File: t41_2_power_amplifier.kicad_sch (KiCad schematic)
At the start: 45 parts, among them J1 5-1814832-1, J2 5-1814832-1, J3 B2B-XH-A_LF__SN_, J5 Screw_Terminal_01x02, Q1 Q_NMOS_GSD, Q3 Q_NMOS_GSD, T1 Transformer_1P_SS, T2 Transformer_1P_1S, U1 MCP1802x-xx02xOT

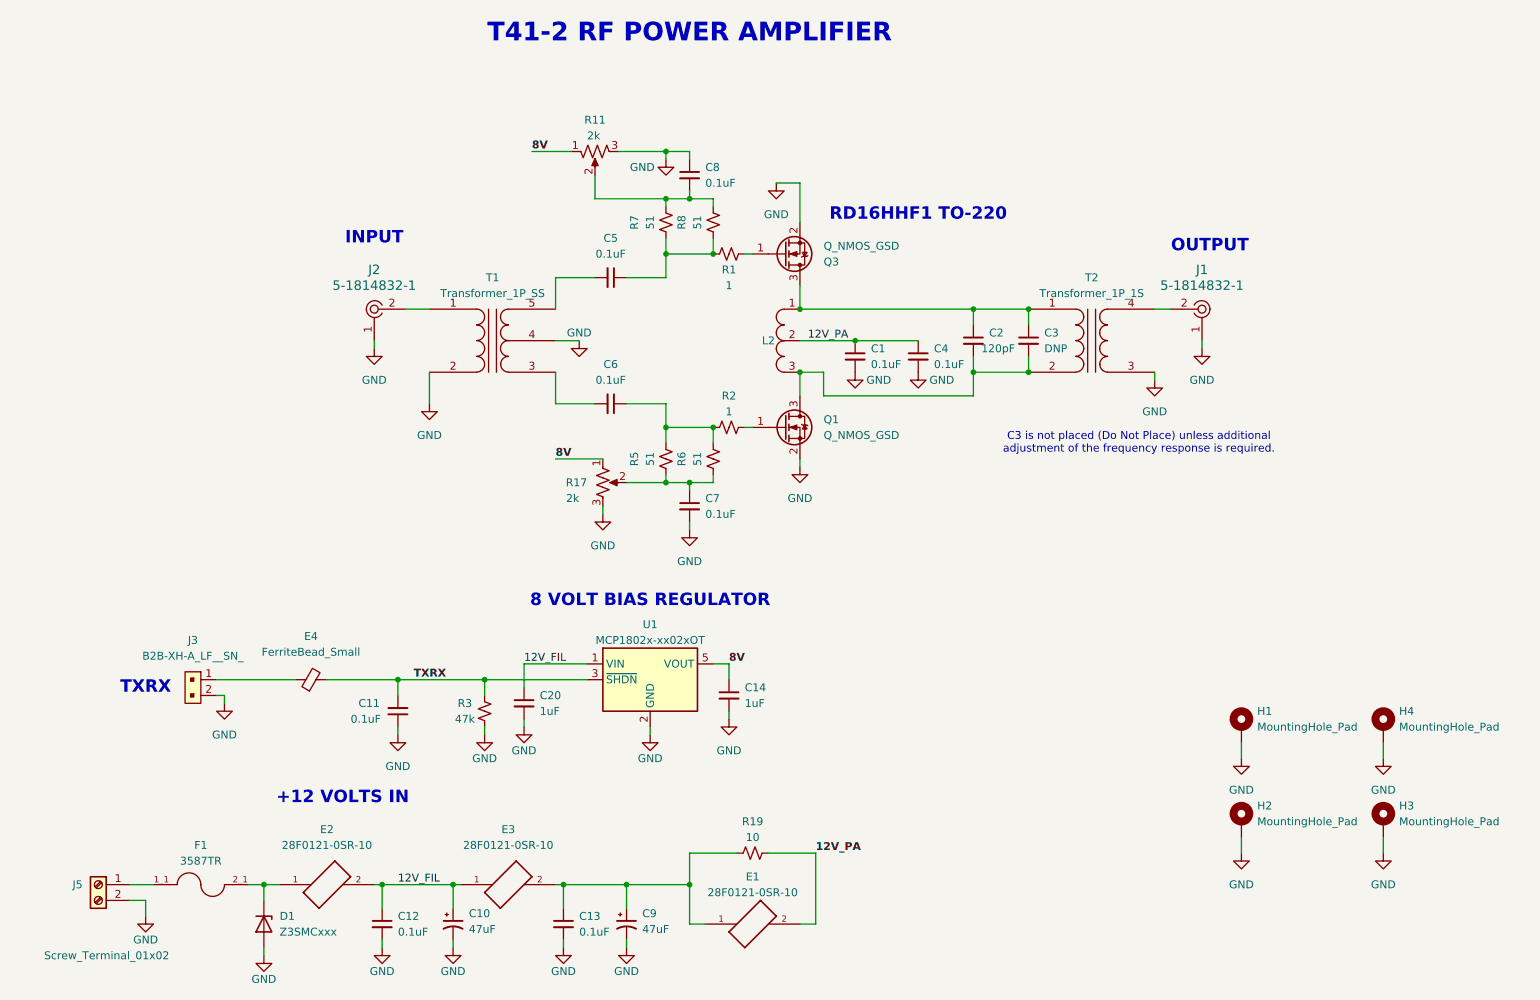
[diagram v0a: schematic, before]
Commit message: Added zip files.
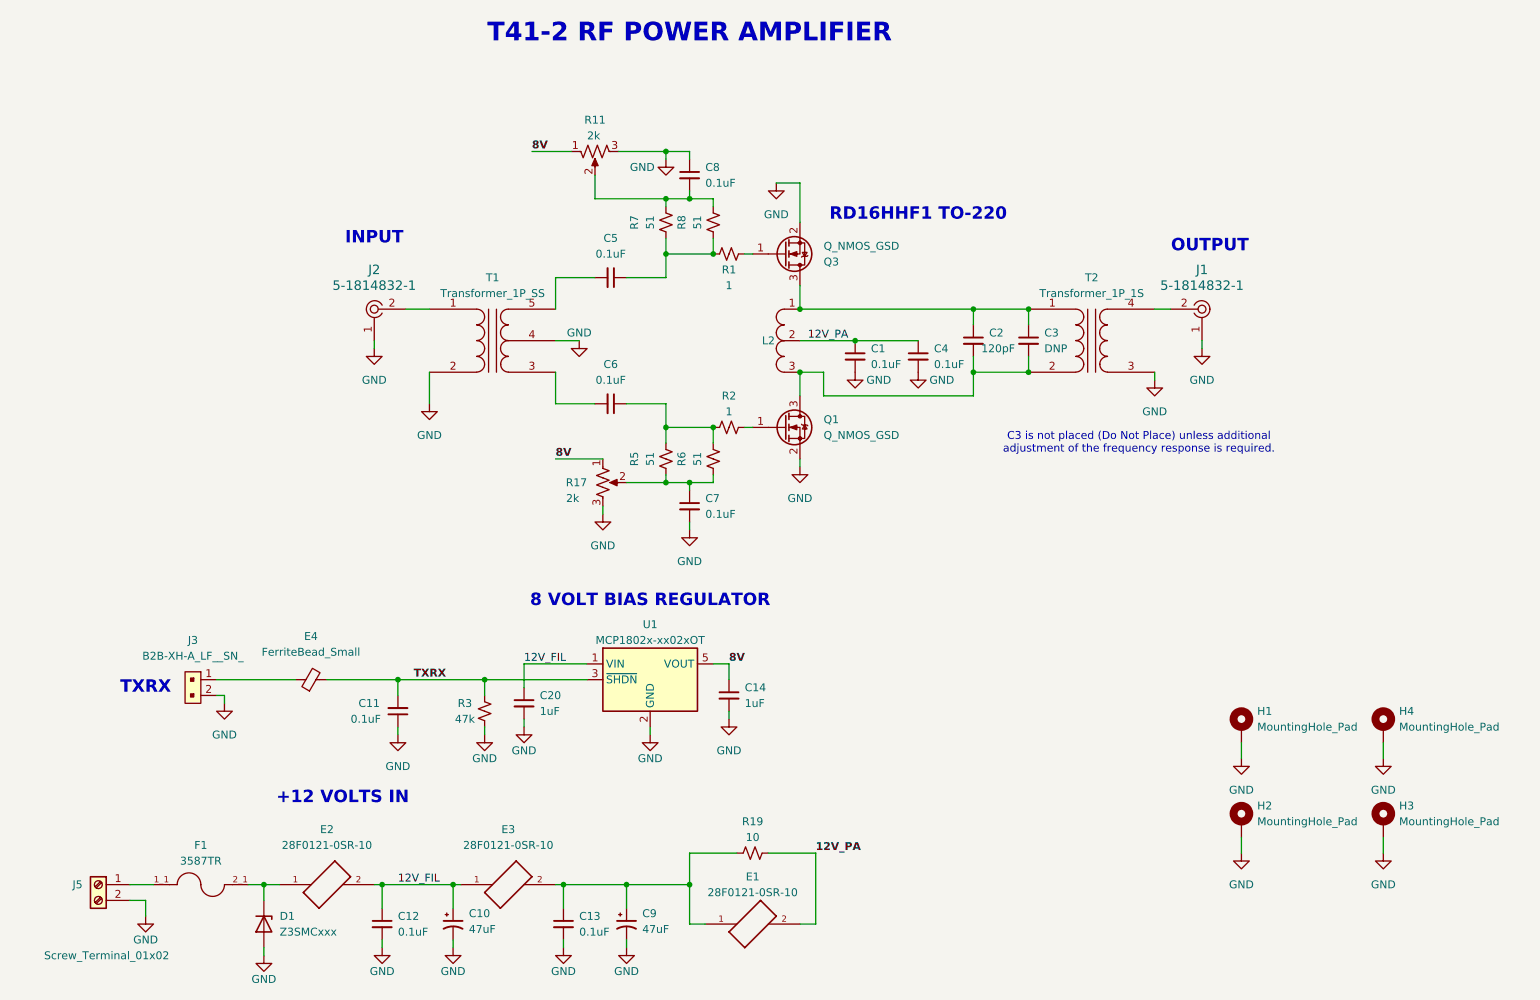
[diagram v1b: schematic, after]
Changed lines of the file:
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@@
 (kicad_sch
-	(version 20231120)
+	(version 20250114)
 	(generator "eeschema")
-	(generator_version "8.0")
+	(generator_version "9.0")
 	(paper "USLetter")
 	(title_block
@@
 		(rev "1.3")
 	)
+	(text "OUTPUT"
+		(exclude_from_sim no)
+		(at 212.09 63.5 0)
+		(effects
+			(font
+				(size 2 2)
+				(thickness 0.4)
+				(bold yes)
+			)
+		)
+	)
+	(text "RD16HHF1 TO-220"
+		(exclude_from_sim no)
+		(at 165.1 58.42 0)
+		(effects
+			(font
+				(size 2 2)
+				(thickness 0.4)
+				(bold yes)
+			)
+		)
+	)
+	(text "+12 VOLTS IN"
+		(exclude_from_sim no)
+		(at 72.39 152.4 0)
+		(effects
+			(font
+				(size 2 2)
+				(thickness 0.4)
+				(bold yes)
+			)
+		)
+	)
+	(text "TXRX"
+		(exclude_from_sim no)
+		(at 40.64 134.62 0)
+		(effects
+			(font
+				(size 2 2)
+				(thickness 0.4)
+				(bold yes)
+			)
+		)
+	)
+	(text "T41-2 RF POWER AMPLIFIER"
+		(exclude_from_sim no)
+		(at 128.27 29.21 0)
+		(effects
+			(font
+				(size 3 3)
+				(thickness 0.6)
+				(bold yes)
+			)
+		)
+	)
+	(text "INPUT"
+		(exclude_from_sim no)
+		(at 77.47 62.23 0)
+		(effects
+			(font
+				(size 2 2)
+				(thickness 0.4)
+				(bold yes)
+			)
+		)
+	)
+	(text "C3 is not placed (Do Not Place) unless additional\nadjustment of the frequency response is required."
+		(exclude_from_sim no)
+		(at 200.66 95.25 0)
+		(effects
+			(font
+				(size 1.27 1.27)
+			)
+		)
+	)
+	(text "8 VOLT BIAS REGULATOR"
+		(exclude_from_sim no)
+		(at 121.92 120.65 0)
+		(effects
+			(font
+				(size 2 2)
+				(thickness 0.4)
+				(bold yes)
+			)
+		)
+	)
 	(junction
 		(at 78.74 166.37)
@@
 		)
 	)
-	(text "OUTPUT"
-		(exclude_from_sim no)
-		(at 212.09 63.5 0)
-		(effects
-			(font
-				(size 2 2)
-				(thickness 0.4)
-				(bold yes)
-			)
-		)
-	)
-	(text "RD16HHF1 TO-220"
-		(exclude_from_sim no)
-		(at 165.1 58.42 0)
-		(effects
-			(font
-				(size 2 2)
-				(thickness 0.4)
-				(bold yes)
-			)
-		)
-	)
-	(text "+12 VOLTS IN"
-		(exclude_from_sim no)
-		(at 72.39 152.4 0)
-		(effects
-			(font
-				(size 2 2)
-				(thickness 0.4)
-				(bold yes)
-			)
-		)
-	)
-	(text "TXRX"
-		(exclude_from_sim no)
-		(at 40.64 134.62 0)
-		(effects
-			(font
-				(size 2 2)
-				(thickness 0.4)
-				(bold yes)
-			)
-		)
-	)
-	(text "T41-2 RF POWER AMPLIFIER"
-		(exclude_from_sim no)
-		(at 128.27 29.21 0)
-		(effects
-			(font
-				(size 3 3)
-				(thickness 0.6)
-				(bold yes)
-			)
-		)
-	)
-	(text "INPUT"
-		(exclude_from_sim no)
-		(at 77.47 62.23 0)
-		(effects
-			(font
-				(size 2 2)
-				(thickness 0.4)
-				(bold yes)
-			)
-		)
-	)
-	(text "C3 is not placed (Do Not Place) unless additional\nadjustment of the frequency response is required."
-		(exclude_from_sim no)
-		(at 200.66 95.25 0)
-		(effects
-			(font
-				(size 1.27 1.27)
-			)
-		)
-	)
-	(text "8 VOLT BIAS REGULATOR"
-		(exclude_from_sim no)
-		(at 121.92 120.65 0)
-		(effects
-			(font
-				(size 2 2)
-				(thickness 0.4)
-				(bold yes)
-			)
-		)
-	)
 	(label "8V"
 		(at 106.68 97.79 0)
@@
 		)
 	)
+	(embedded_fonts no)
 )
